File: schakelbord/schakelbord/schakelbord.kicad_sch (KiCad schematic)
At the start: 113 parts, among them J1 Screw_Terminal_01x03, J12 I/O nano, J15 Relais 7&8, J16 Alalog i/o, J17 Extra 1-4, J18 Extra 5-8, J19 Relais 5&6, J20 Relais 3&4, J21 Relais 1&2, J3 Power, J4 mosfets, K10 SANYOU_SRD_Form_C, K3 SANYOU_SRD_Form_C, K4 SANYOU_SRD_Form_C, K5 SANYOU_SRD_Form_C, K6 SANYOU_SRD_Form_C, K7 SANYOU_SRD_Form_C, K8 SANYOU_SRD_Form_C, K9 SANYOU_SRD_Form_C, Q1 BC337, Q10 BC337, Q11 BC337, Q12 BC337, Q13 BC337, Q14 BC337, Q15 IRLZ44N, Q2 IRLZ44N, Q3 IRLZ44N, Q5 BC337, Q6 BC337, Q9 BC337, U1 MCP23017x-x-SP

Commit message: pcb update
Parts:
- C1: footprint PCM_SparkFun-Capacitor:C_0402_1005Metric -> Capacitor_THT:C_Disc_D3.0mm_W1.6mm_P2.50mm
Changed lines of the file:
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@@
 			)
 		)
-		(property "Footprint" "PCM_SparkFun-Capacitor:C_0402_1005Metric"
+		(property "Footprint" "Capacitor_THT:C_Disc_D3.0mm_W1.6mm_P2.50mm"
 			(at 234.95 337.82 0)
 			(hide yes)

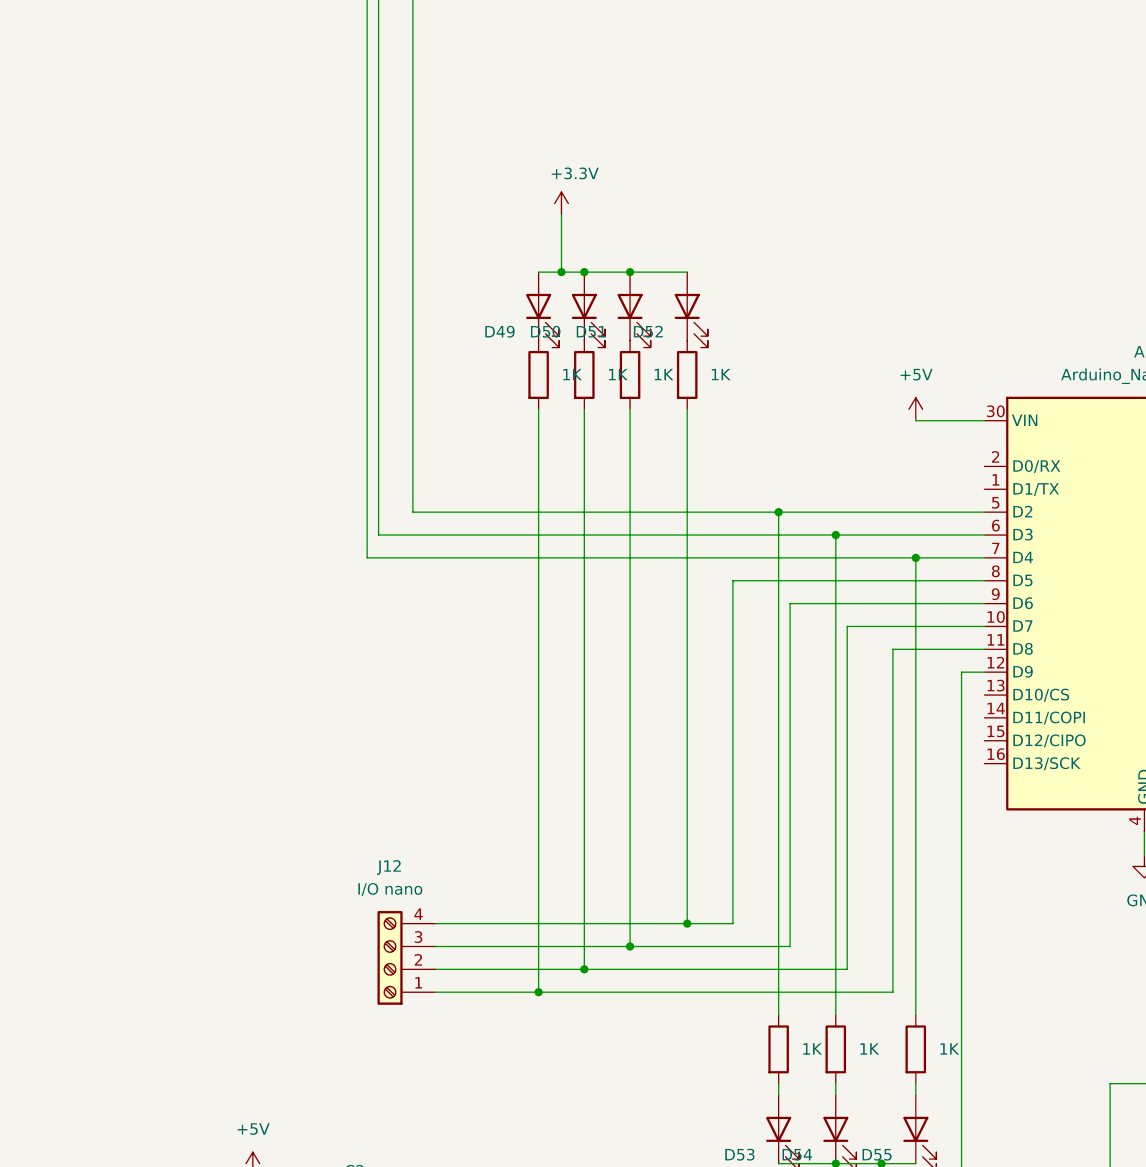
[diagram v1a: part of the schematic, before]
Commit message: pcb update
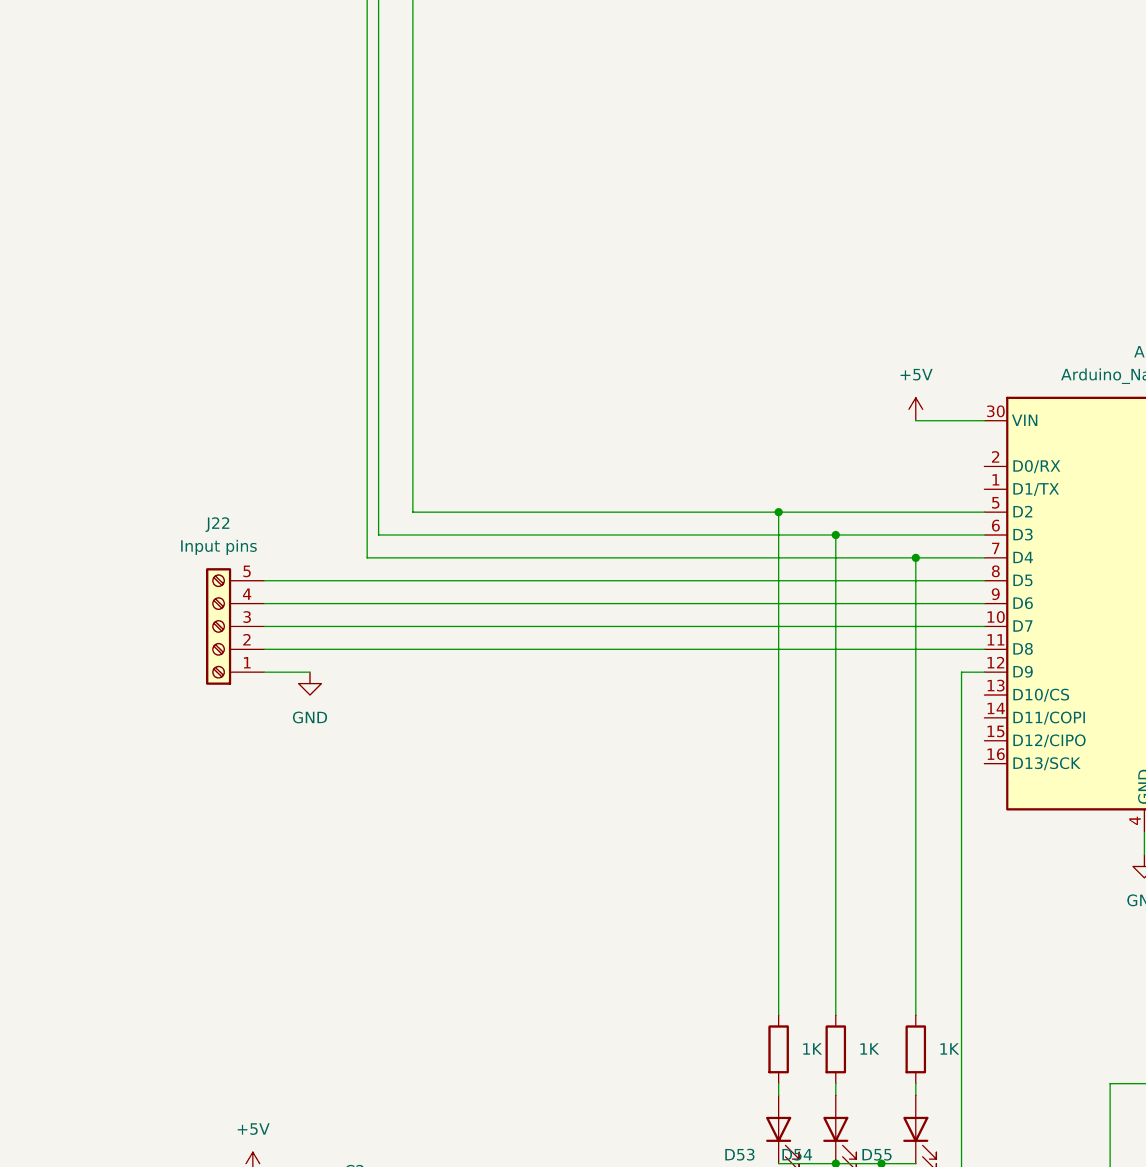
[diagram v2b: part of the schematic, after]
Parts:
- removed D49, D50, D51, D52: LED, LED_THT:LED_D5.0mm, symbol Device:LED
- removed J12: I/O nano, TerminalBlock_Phoenix:TerminalBlock_Phoenix_MKDS-1,5-4-5.08_1x04_P5.08mm_Horizontal, symbol Connector:Screw_Terminal_01x04
- removed R63, R64, R65, R66: 1K, Resistor_THT:R_Axial_DIN0204_L3.6mm_D1.6mm_P7.62mm_Horizontal, symbol Device:R
- added J22: Input pins, TerminalBlock_Phoenix:TerminalBlock_Phoenix_MKDS-1,5-5-5.08_1x05_P5.08mm_Horizontal, symbol Connector:Screw_Terminal_01x05
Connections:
- net GND: now also J22.1 (Pin_1)
- net at A1.10 (D7): now also J22.3 (Pin_3)
- net at A1.11 (D8): now also J22.2 (Pin_2)
- net at A1.8 (D5): now also J22.5 (Pin_5)
- net at A1.9 (D6): now also J22.4 (Pin_4)

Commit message: pcb update
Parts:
- C1: footprint Capacitor_THT:C_Disc_D3.0mm_W1.6mm_P2.50mm -> Capacitor_THT:C_Disc_D5.0mm_W2.5mm_P5.00mm
- C2: footprint PCM_SparkFun-Capacitor:Electrolytic_10.3x10.3mm -> Capacitor_THT:CP_Radial_D8.0mm_P3.50mm
- Q1, Q10, Q11, Q12, Q13, Q14, Q5, Q6, Q9: footprint Package_TO_SOT_THT:TO-92_Inline -> Package_TO_SOT_THT:TO-92L_Inline_Wide
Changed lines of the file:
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@@
 			)
 		)
-		(property "Footprint" "Package_TO_SOT_THT:TO-92_Inline"
+		(property "Footprint" "Package_TO_SOT_THT:TO-92L_Inline_Wide"
 			(at 180.34 365.125 0)
 			(hide yes)
@@
 			)
 		)
-		(property "Footprint" "Package_TO_SOT_THT:TO-92_Inline"
+		(property "Footprint" "Package_TO_SOT_THT:TO-92L_Inline_Wide"
 			(at 355.6 197.485 0)
 			(hide yes)
@@
 			)
 		)
-		(property "Footprint" "Package_TO_SOT_THT:TO-92_Inline"
+		(property "Footprint" "Package_TO_SOT_THT:TO-92L_Inline_Wide"
 			(at 356.87 140.335 0)
 			(hide yes)
@@
 			)
 		)
-		(property "Footprint" "Package_TO_SOT_THT:TO-92_Inline"
+		(property "Footprint" "Package_TO_SOT_THT:TO-92L_Inline_Wide"
 			(at 410.21 309.245 0)
 			(hide yes)
@@
 			)
 		)
-		(property "Footprint" "Package_TO_SOT_THT:TO-92_Inline"
+		(property "Footprint" "Package_TO_SOT_THT:TO-92L_Inline_Wide"
 			(at 411.48 196.215 0)
 			(hide yes)
@@
 			)
 		)
-		(property "Footprint" "Package_TO_SOT_THT:TO-92_Inline"
+		(property "Footprint" "Package_TO_SOT_THT:TO-92L_Inline_Wide"
 			(at 411.48 253.365 0)
 			(hide yes)
@@
 			)
 		)
-		(property "Footprint" "Package_TO_SOT_THT:TO-92_Inline"
+		(property "Footprint" "Package_TO_SOT_THT:TO-92L_Inline_Wide"
 			(at 412.75 139.065 0)
 			(hide yes)
@@
 			)
 		)
-		(property "Footprint" "Capacitor_THT:C_Disc_D3.0mm_W1.6mm_P2.50mm"
+		(property "Footprint" "Capacitor_THT:C_Disc_D5.0mm_W2.5mm_P5.00mm"
 			(at 234.95 337.82 0)
 			(hide yes)
@@
 			)
 		)
-		(property "Footprint" "Package_TO_SOT_THT:TO-92_Inline"
+		(property "Footprint" "Package_TO_SOT_THT:TO-92L_Inline_Wide"
 			(at 355.6 254.635 0)
 			(hide yes)
@@
 			)
 		)
-		(property "Footprint" "PCM_SparkFun-Capacitor:Electrolytic_10.3x10.3mm"
+		(property "Footprint" "Capacitor_THT:CP_Radial_D8.0mm_P3.50mm"
 			(at 59.69 378.46 0)
 			(hide yes)
@@
 			)
 		)
-		(property "Footprint" "Package_TO_SOT_THT:TO-92_Inline"
+		(property "Footprint" "Package_TO_SOT_THT:TO-92L_Inline_Wide"
 			(at 354.33 310.515 0)
 			(hide yes)
